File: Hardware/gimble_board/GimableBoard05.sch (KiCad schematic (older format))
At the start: 38 parts, among them Q1 Q_NMOS_GDS, Q2 Q_NMOS_GDS, Q3 Q_NMOS_GDS, Q4 Q_NMOS_GDS, Q5 Q_NMOS_GDS, Q6 Q_NMOS_GDS, Q7 Q_NMOS_GDS, Q8 Q_NMOS_GDS

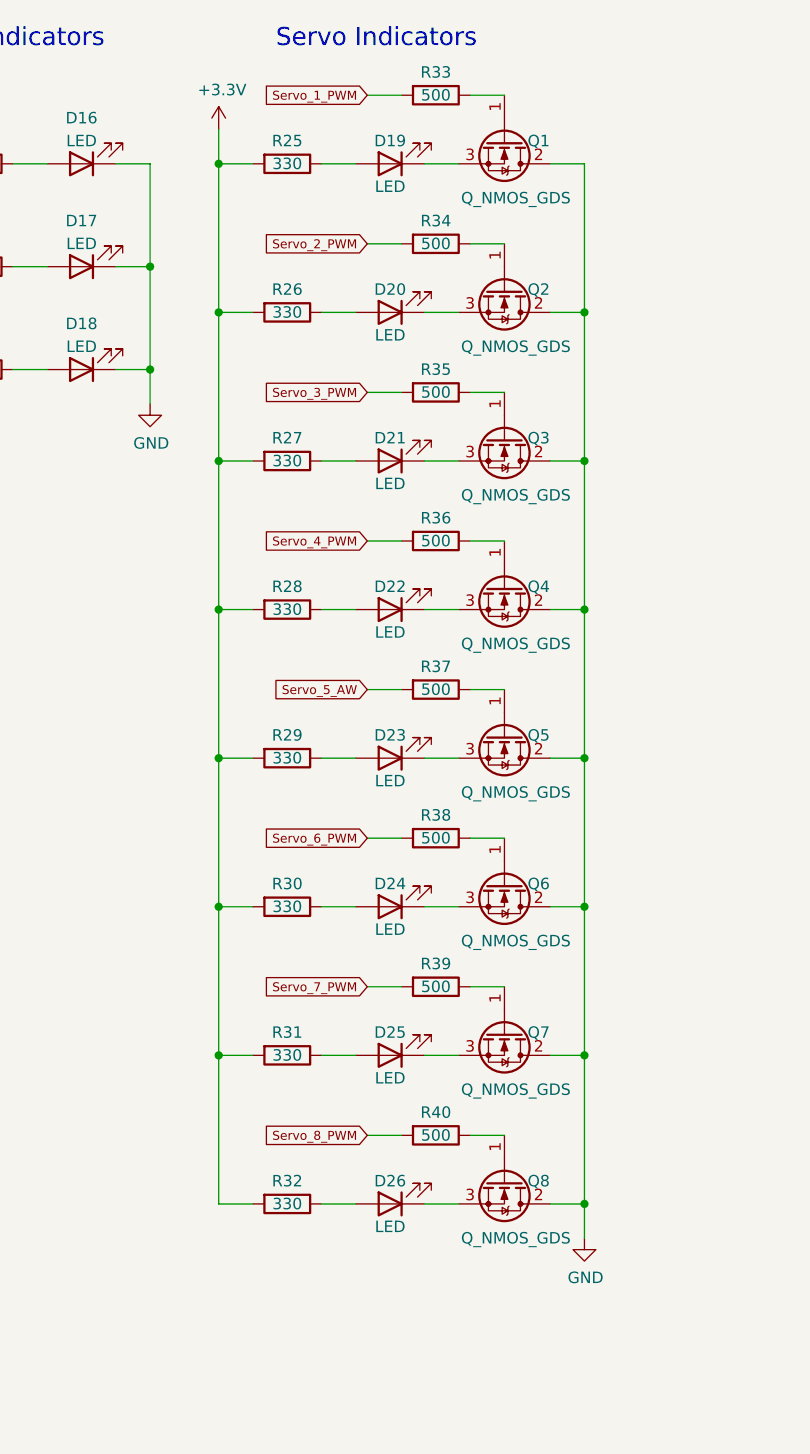
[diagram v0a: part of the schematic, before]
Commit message: Fixed MOSFET's
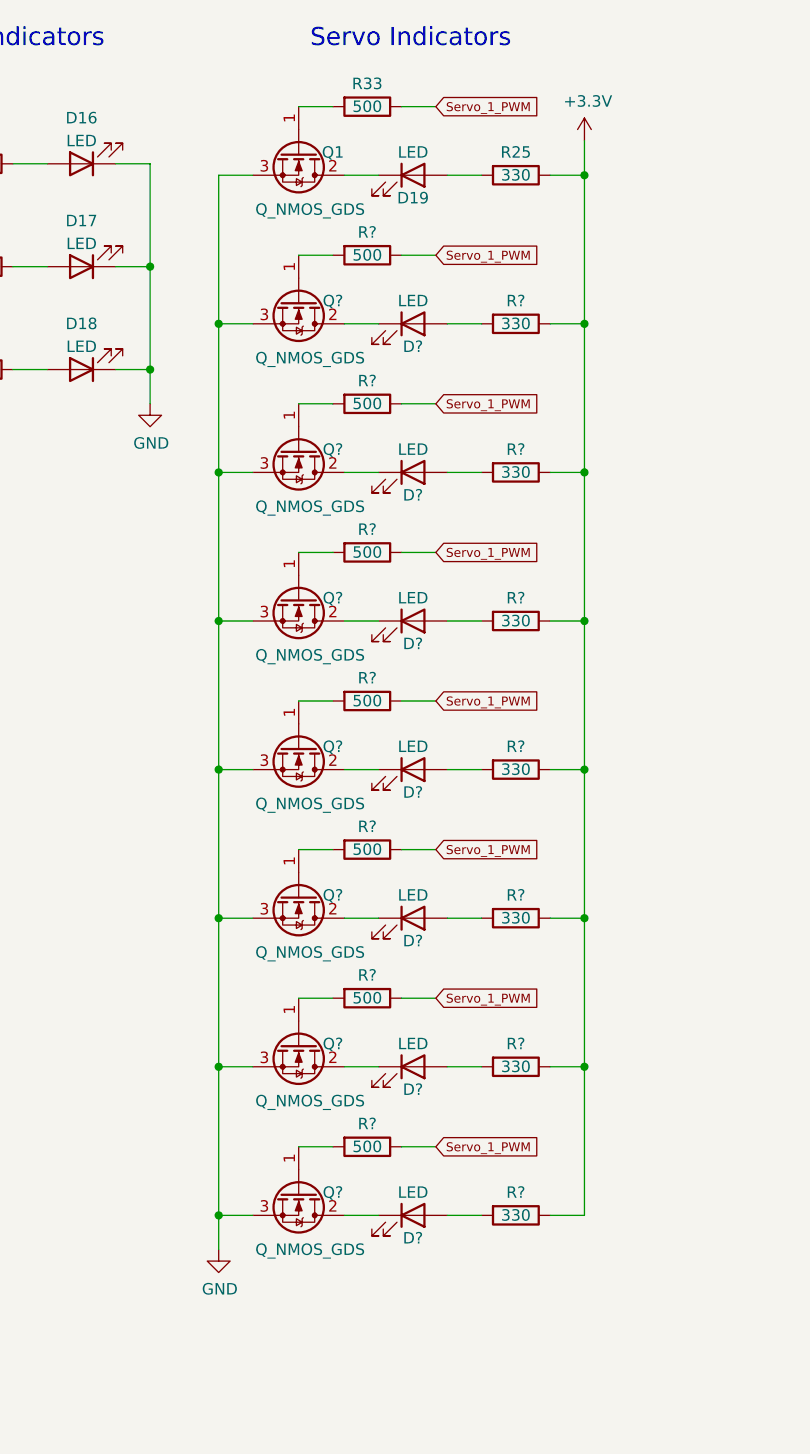
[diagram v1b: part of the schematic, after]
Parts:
- removed D20, D21, D22, D23, D24, D25, D26: LED, symbol Device:LED
- removed Q2, Q3, Q4, Q5, Q6, Q7, Q8: Q_NMOS_GDS, symbol Device:Q_NMOS_GDS
- removed R26, R27, R28, R29, R30, R31, R32: 330, symbol Device:R
- removed R34, R35, R36, R37, R38, R39, R40: 500, symbol Device:R
- added D? (x7): LED, symbol Device:LED
- added Q? (x7): Q_NMOS_GDS, symbol Device:Q_NMOS_GDS
- added R? (x7): 330, symbol Device:R
- added R? (x7): 500, symbol Device:R
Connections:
- net +3V3: now also R25.1, R?.1, R?.1, R?.1, R?.1, R?.1, R?.1, R?.1; no longer R25.2
- net GND: now also Q1.3 (S), Q?.3 (S), Q?.3 (S), Q?.3 (S), Q?.3 (S), Q?.3 (S), Q?.3 (S), Q?.3 (S); no longer Q1.2 (D)
- net Servo_1_PWM: now also R33.1, R?.1, R?.1, R?.1, R?.1, R?.1, R?.1, R?.1; no longer R33.2
- net at D19.2 (A): now also R25.2; no longer R25.1
- net at D19.1 (K): now also Q1.2 (D); no longer Q1.3 (S)
- net at Q1.1 (G): now also R33.2; no longer R33.1
- new net: D?.2 (A), R?.2 (x7)
- new net: D?.1 (K), Q?.2 (D) (x7)
- new net: Q?.1 (G), R?.2 (x7)
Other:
- moved on the sheet: D19, Q1, R25, R33
